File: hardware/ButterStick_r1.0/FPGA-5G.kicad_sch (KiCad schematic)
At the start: 1 part, among them U4 ECP5UM5G_85_CABGA381

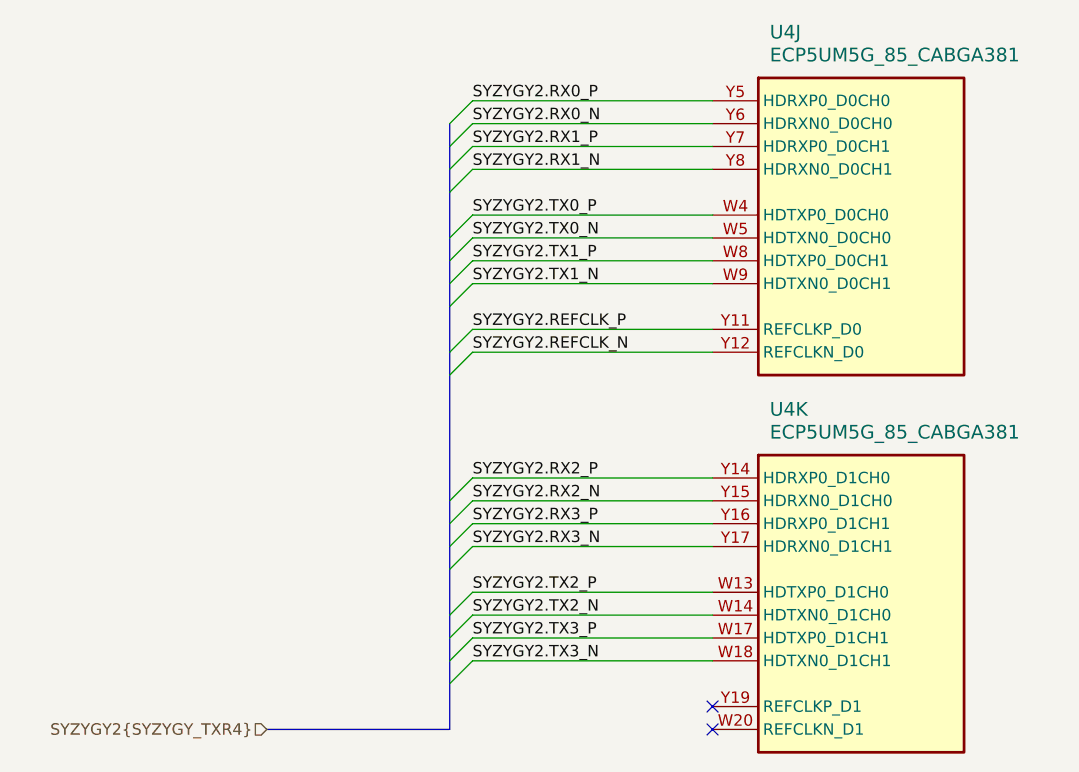
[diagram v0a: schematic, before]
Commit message: hw.r1d0: Review complete, gerbers generated
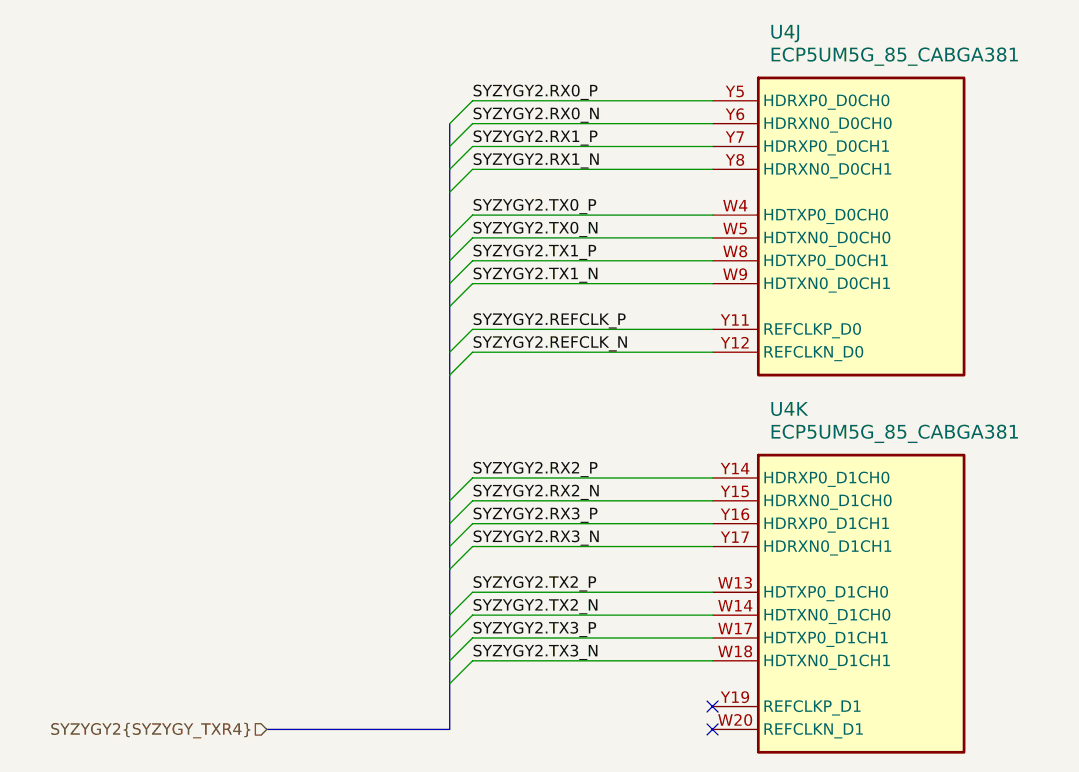
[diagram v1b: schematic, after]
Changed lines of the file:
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@@
 (kicad_sch (version 20200618) (host eeschema "5.99.0-unknown-73168a9~101~ubuntu18.04.1")
-  (page 11 18)
+  (page 1 18)
   (paper "A4")
   (title_block
     (title "ButterStick")
-    (date "2020-07-16")
+    (date "2020-07-17")
     (rev "r1.0")
     (company "GsD")
     (comment 1 "Functional prototyping board for the Lattice ECP5.")
   )
+  (no_connect (at 119.38 134.62))
   (no_connect (at 119.38 132.08))
-  (no_connect (at 119.38 134.62))
   (bus_entry (at 90.17 67.31) (size 2.54 -2.54)
     (stroke (width 0.1524) (type solid) (color 0 0 0 0))
@@
     (stroke (width 0) (type solid) (color 0 0 0 0))
   )
-  (bus (pts (xy 90.17 67.31) (xy 90.17 69.85))
+  (bus (pts (xy 90.17 67.31) (xy 90.17 72.39))
     (stroke (width 0) (type solid) (color 0 0 0 0))
   )
-  (bus (pts (xy 90.17 69.85) (xy 90.17 74.93))
+  (bus (pts (xy 90.17 72.39) (xy 90.17 80.01))
     (stroke (width 0) (type solid) (color 0 0 0 0))
   )
-  (bus (pts (xy 90.17 74.93) (xy 90.17 82.55))
+  (bus (pts (xy 90.17 80.01) (xy 90.17 82.55))
     (stroke (width 0) (type solid) (color 0 0 0 0))
   )
@@
     (stroke (width 0) (type solid) (color 0 0 0 0))
   )
-  (bus (pts (xy 90.17 87.63) (xy 90.17 92.71))
+  (bus (pts (xy 90.17 87.63) (xy 90.17 95.25))
     (stroke (width 0) (type solid) (color 0 0 0 0))
   )
-  (bus (pts (xy 90.17 92.71) (xy 90.17 109.22))
+  (bus (pts (xy 90.17 95.25) (xy 90.17 111.76))
     (stroke (width 0) (type solid) (color 0 0 0 0))
   )
-  (bus (pts (xy 90.17 109.22) (xy 90.17 114.3))
+  (bus (pts (xy 90.17 111.76) (xy 90.17 116.84))
     (stroke (width 0) (type solid) (color 0 0 0 0))
   )
-  (bus (pts (xy 90.17 114.3) (xy 90.17 121.92))
+  (bus (pts (xy 90.17 116.84) (xy 90.17 121.92))
     (stroke (width 0) (type solid) (color 0 0 0 0))
   )
